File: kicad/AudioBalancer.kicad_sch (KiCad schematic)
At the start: 25 parts, among them J1 Conn_01x03_Pin, J2 Conn_01x03_Pin, J3 Conn_01x02_Pin, J4 Conn_01x02_Pin, J5 Conn_01x03_Pin, U1 SSM2141, U2 SSM2142P

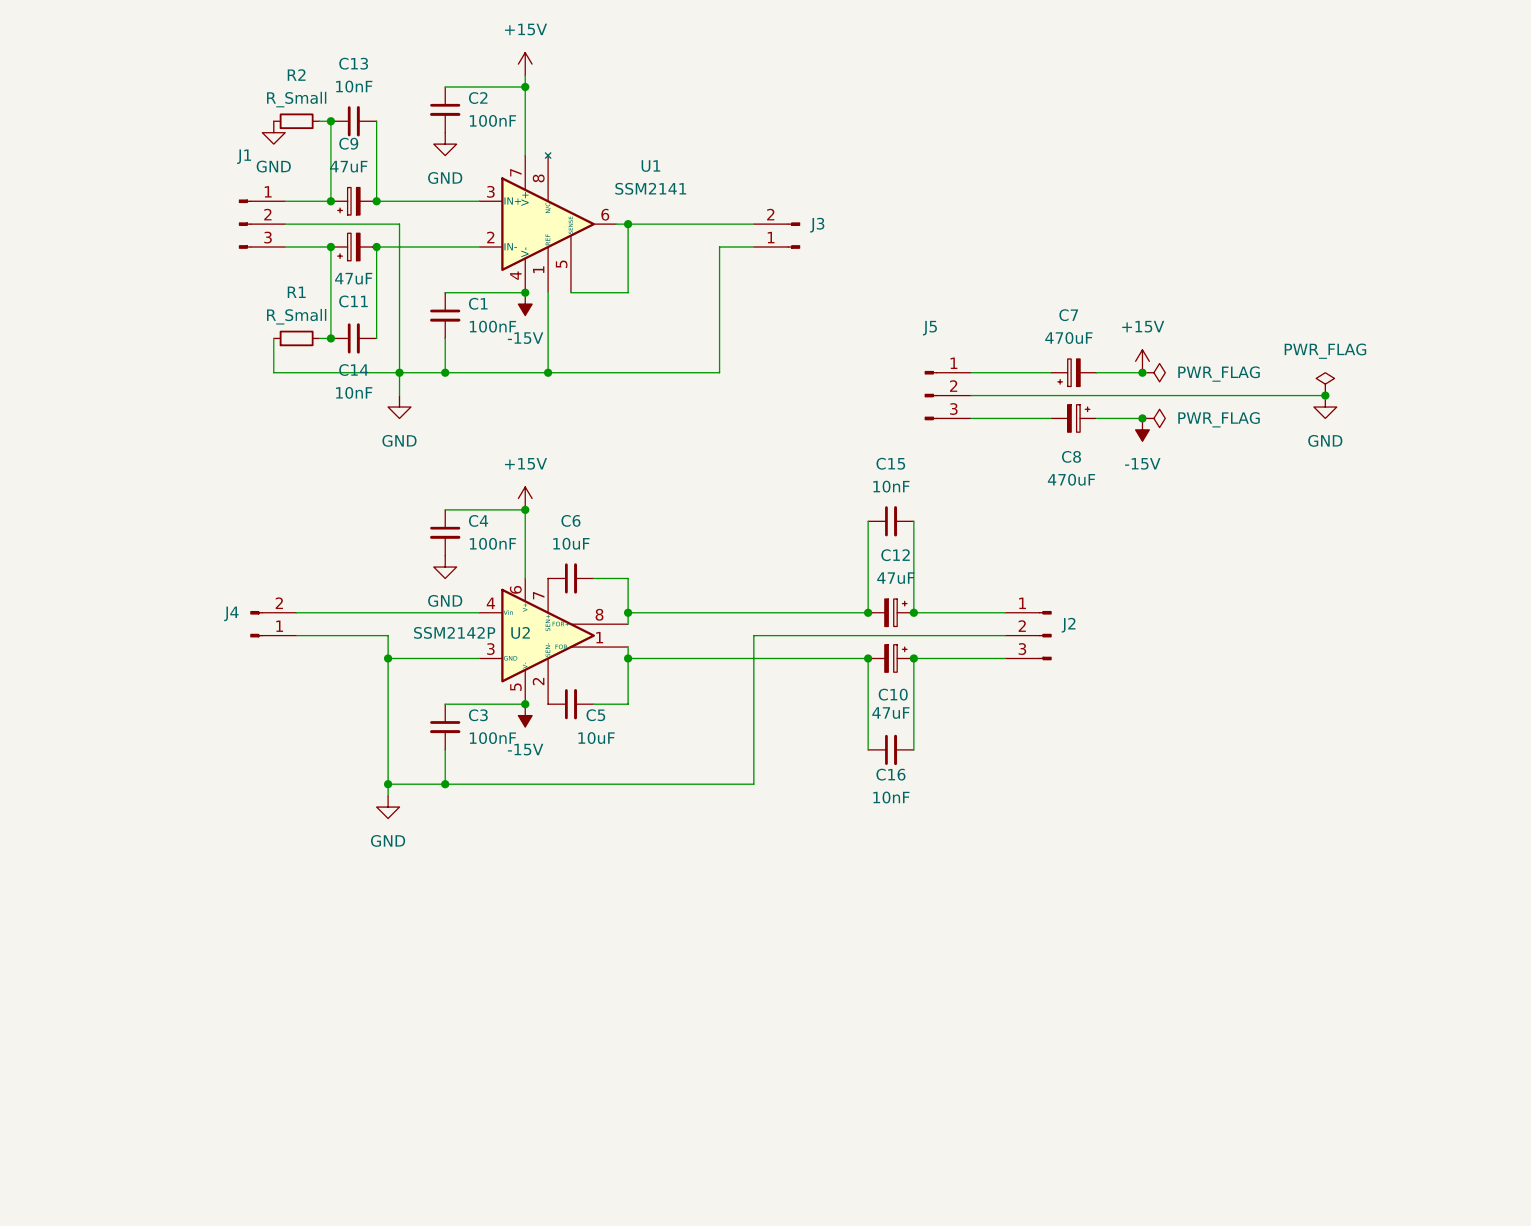
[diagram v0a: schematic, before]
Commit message: Completed V1.0
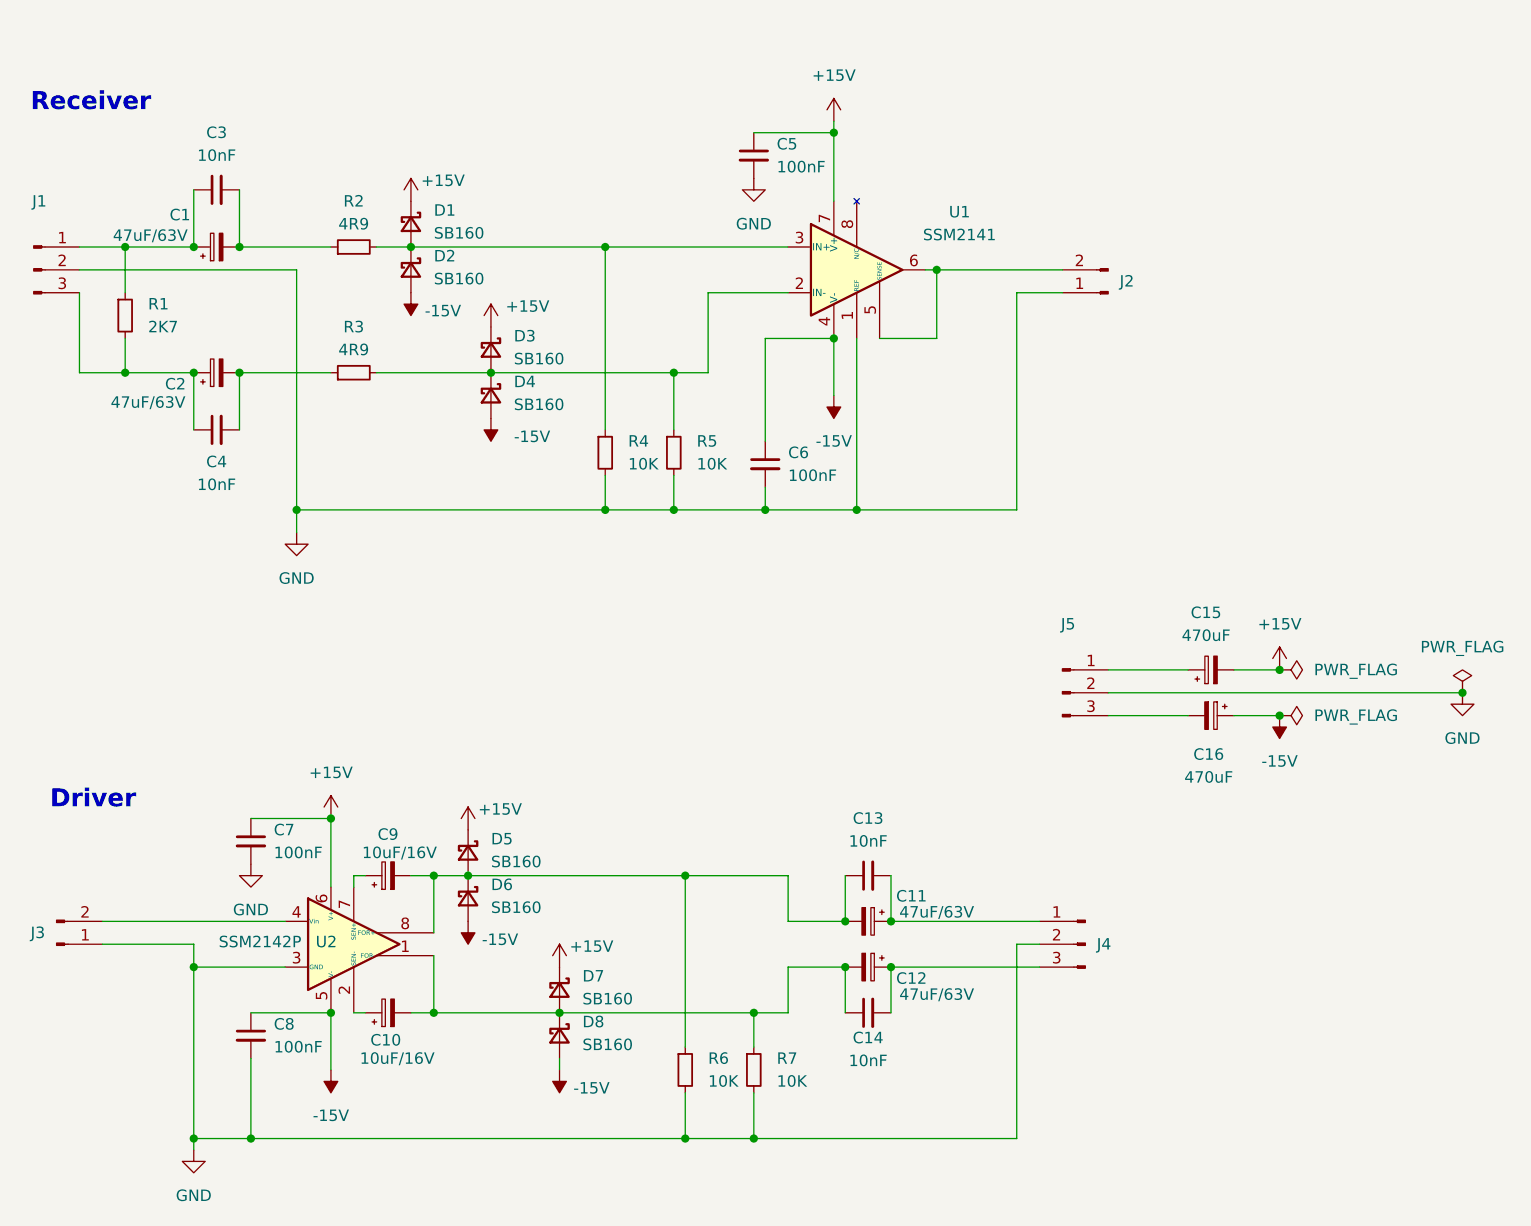
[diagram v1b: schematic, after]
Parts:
- removed C5, C6: 10uF, symbol Device:C_Small
- added C10, C9: 10uF/16V, Capacitor_THT:CP_Radial_D5.0mm_P2.00mm, symbol Device:C_Polarized_Small
- added D1, D2, D3, D4, D5, D6, D7, D8: SB160, Diode_THT:D_DO-41_SOD81_P10.16mm_Horizontal, symbol Device:D_Schottky_Small
- added R3: 4R9, Resistor_THT:R_Axial_DIN0207_L6.3mm_D2.5mm_P10.16mm_Horizontal, symbol Device:R_Small
- added R4, R5, R6, R7: 10K, Resistor_THT:R_Axial_DIN0207_L6.3mm_D2.5mm_P10.16mm_Horizontal, symbol Device:R_Small
- C1: renamed from C9; value 47uF -> 47uF/63V; footprint (none) -> Capacitor_THT:CP_Radial_D10.0mm_P5.00mm
- C11: renamed from C12; value 47uF -> 47uF/63V; footprint (none) -> Capacitor_THT:CP_Radial_D10.0mm_P5.00mm
- C12: renamed from C10; value 47uF -> 47uF/63V; footprint (none) -> Capacitor_THT:CP_Radial_D10.0mm_P5.00mm
- C13: renamed from C15; footprint (none) -> Capacitor_THT:C_Rect_L7.0mm_W2.0mm_P5.00mm
- C14: renamed from C16; footprint (none) -> Capacitor_THT:C_Rect_L7.0mm_W2.0mm_P5.00mm
- C15: renamed from C7; footprint (none) -> Capacitor_THT:CP_Radial_D10.0mm_P5.00mm_P7.50mm
- C16: renamed from C8; footprint (none) -> Capacitor_THT:CP_Radial_D10.0mm_P5.00mm_P7.50mm
- C2: renamed from C11; value 47uF -> 47uF/63V; footprint (none) -> Capacitor_THT:CP_Radial_D10.0mm_P5.00mm
- C3: renamed from C13; footprint (none) -> Capacitor_THT:C_Rect_L7.0mm_W2.0mm_P5.00mm
- C4: renamed from C14; footprint (none) -> Capacitor_THT:C_Rect_L7.0mm_W2.0mm_P5.00mm
- C5: renamed from C2; footprint (none) -> Capacitor_THT:C_Rect_L7.0mm_W2.5mm_P5.00mm
- C6: renamed from C1; footprint (none) -> Capacitor_THT:C_Rect_L7.0mm_W2.5mm_P5.00mm
- C7: renamed from C4; footprint (none) -> Capacitor_THT:C_Rect_L7.0mm_W2.5mm_P5.00mm
- C8: renamed from C3; footprint (none) -> Capacitor_THT:C_Rect_L7.0mm_W2.5mm_P5.00mm
- J1, J5: footprint (none) -> Connector_Molex:Molex_KK-254_AE-6410-03A_1x03_P2.54mm_Vertical
- J2: renamed from J3; footprint (none) -> Connector_Molex:Molex_KK-254_AE-6410-02A_1x02_P2.54mm_Vertical
- J3: renamed from J4; footprint (none) -> Connector_Molex:Molex_KK-254_AE-6410-02A_1x02_P2.54mm_Vertical
- J4: renamed from J2; footprint (none) -> Connector_Molex:Molex_KK-254_AE-6410-03A_1x03_P2.54mm_Vertical
- R1: value R_Small -> 2K7; footprint (none) -> Resistor_THT:R_Axial_DIN0207_L6.3mm_D2.5mm_P10.16mm_Horizontal
- R2: value R_Small -> 4R9; footprint (none) -> Resistor_THT:R_Axial_DIN0207_L6.3mm_D2.5mm_P10.16mm_Horizontal
- U1, U2: footprint (none) -> Package_DIP:DIP-8_W7.62mm
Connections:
- net +15V: now also D1.1 (K), D3.1 (K), D5.1 (K), D7.1 (K)
- net -15V: now also D2.2 (A), D4.2 (A), D6.2 (A), D8.2 (A)
- net GND: now also R4.2, R5.2, R6.2, R7.2; no longer R1.1, R2.1
- net at C11.2, C13.1, U2.8 (FOR+): now also C9.2, D5.2 (A), D6.1 (K), R6.1
- net at C12.2, C14.1, U2.1 (FOR-): now also C10.2, D7.2 (A), D8.1 (K), R7.1
- net at U2.2 (SEN-): now also C10.1
- net at U2.7 (SEN+): now also C9.1
- net at C2.2, C4.2: now also R3.1; no longer U1.2 (IN-)
- net at C1.1, C3.1, J1.1 (Pin_1): now also R1.1; no longer R2.2
- net at C1.2, C3.2: now also R2.1; no longer U1.3 (IN+)
- new net: D1.2 (A), D2.1 (K), R2.2, R4.1, U1.3 (IN+)
- new net: D3.2 (A), D4.1 (K), R3.2, R5.1, U1.2 (IN-)
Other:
- note added: "Driver"
- note added: "Receiver"
- moved on the sheet: C1, C11, C12, C13, C14, C15, C16, C2, C3, C4, C5, C6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
